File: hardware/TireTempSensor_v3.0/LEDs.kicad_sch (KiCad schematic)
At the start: 10 parts

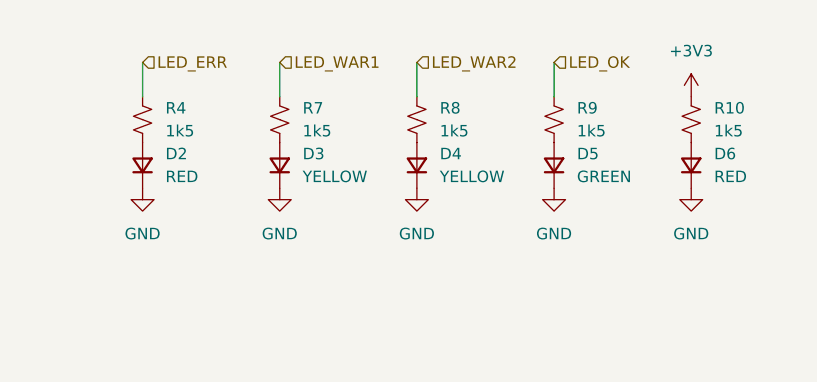
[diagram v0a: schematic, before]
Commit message: Propozycja layoutu na spotkanie
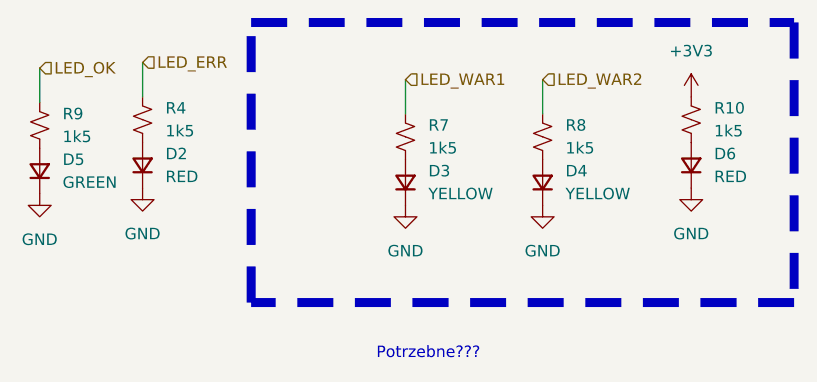
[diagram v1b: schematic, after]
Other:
- note added: "Potrzebne???"
- moved on the sheet: D3, D4, D5, R7, R8, R9
